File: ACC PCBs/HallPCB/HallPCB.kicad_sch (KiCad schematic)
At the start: 2 parts, among them J1 Conn_01x04_Socket, U1 TLE49643MXTMA1

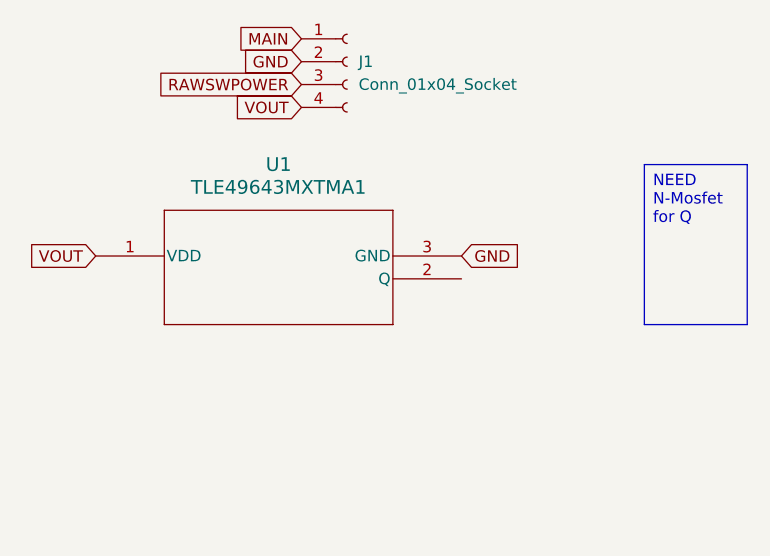
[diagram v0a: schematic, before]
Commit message: All boards should be finished. ACC otw, and an earlier version of the main board otw
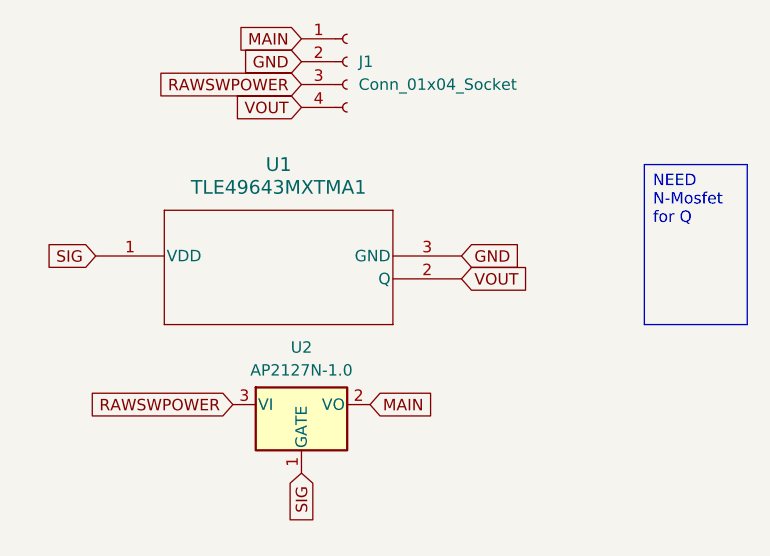
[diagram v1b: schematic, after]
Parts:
- added U2: AP2127N-1.0, Package_TO_SOT_SMD:SOT-23, symbol Regulator_Linear:AP2127N-1.0
- J1: footprint (none) -> Connector_PinHeader_2.54mm:PinHeader_1x04_P2.54mm_Horizontal
- U1: footprint PG-SOT23-3-15_INF -> TLE49643MXTMA1:PG-SOT23-3-15_INF
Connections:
- net MAIN: now also U2.2 (VO)
- net RAWSWPOWER: now also U2.3 (VI)
- net VOUT: now also U1.2 (Q); no longer U1.1 (VDD)
- new net SIG: U1.1 (VDD), U2.1 (GATE)
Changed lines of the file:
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@@
 	(global_label "VOUT"
 		(shape input)
+		(at 160.02 107.95 0)
+		(fields_autoplaced yes)
+		(effects
+			(font
+				(size 1.27 1.27)
+			)
+			(justify left)
+		)
+		(property "Intersheetrefs" "${INTERSHEET_REFS}"
+			(at 167.7224 107.95 0)
+			(effects
+				(font
+					(size 1.27 1.27)
+				)
+				(justify left)
+				(hide yes)
+			)
+		)
+	)
+	(global_label "RAWSWPOWER"
+		(shape input)
+		(at 142.24 86.36 180)
+		(fields_autoplaced yes)
+		(effects
+			(font
+				(size 1.27 1.27)
+			)
+			(justify right)
+		)
+		(property "Intersheetrefs" "${INTERSHEET_REFS}"
+			(at 126.313 86.36 0)
+			(effects
+				(font
+					(size 1.27 1.27)
+				)
+				(justify right)
+				(hide yes)
+			)
+		)
+	)
+	(global_label "MAIN"
+		(shape input)
+		(at 149.86 121.92 0)
+		(fields_autoplaced yes)
+		(effects
+			(font
+				(size 1.27 1.27)
+			)
+			(justify left)
+		)
+		(property "Intersheetrefs" "${INTERSHEET_REFS}"
+			(at 157.3205 121.92 0)
+			(effects
+				(font
+					(size 1.27 1.27)
+				)
+				(justify left)
+				(hide yes)
+			)
+		)
+	)
+	(global_label "RAWSWPOWER"
+		(shape input)
+		(at 134.62 121.92 180)
+		(fields_autoplaced yes)
+		(effects
+			(font
+				(size 1.27 1.27)
+			)
+			(justify right)
+		)
+		(property "Intersheetrefs" "${INTERSHEET_REFS}"
+			(at 118.693 121.92 0)
+			(effects
+				(font
+					(size 1.27 1.27)
+				)
+				(justify right)
+				(hide yes)
+			)
+		)
+	)
+	(global_label "MAIN"
+		(shape input)
+		(at 142.24 81.28 180)
+		(fields_autoplaced yes)
+		(effects
+			(font
+				(size 1.27 1.27)
+			)
+			(justify right)
+		)
+		(property "Intersheetrefs" "${INTERSHEET_REFS}"
+			(at 134.7795 81.28 0)
+			(effects
+				(font
+					(size 1.27 1.27)
+				)
+				(justify right)
+				(hide yes)
+			)
+		)
+	)
+	(global_label "VOUT"
+		(shape input)
+		(at 142.24 88.9 180)
+		(fields_autoplaced yes)
+		(effects
+			(font
+				(size 1.27 1.27)
+			)
+			(justify right)
+		)
+		(property "Intersheetrefs" "${INTERSHEET_REFS}"
+			(at 134.5376 88.9 0)
+			(effects
+				(font
+					(size 1.27 1.27)
+				)
+				(justify right)
+				(hide yes)
+			)
+		)
+	)
+	(global_label "GND"
+		(shape input)
+		(at 142.24 83.82 180)
+		(fields_autoplaced yes)
+		(effects
+			(font
+				(size 1.27 1.27)
+			)
+			(justify right)
+		)
+		(property "Intersheetrefs" "${INTERSHEET_REFS}"
+			(at 135.3843 83.82 0)
+			(effects
+				(font
+					(size 1.27 1.27)
+				)
+				(justify right)
+				(hide yes)
+			)
+		)
+	)
+	(global_label "GND"
+		(shape input)
+		(at 160.02 105.41 0)
+		(fields_autoplaced yes)
+		(effects
+			(font
+				(size 1.27 1.27)
+			)
+			(justify left)
+		)
+		(property "Intersheetrefs" "${INTERSHEET_REFS}"
+			(at 166.8757 105.41 0)
+			(effects
+				(font
+					(size 1.27 1.27)
+				)
+				(justify left)
+				(hide yes)
+			)
+		)
+	)
+	(global_label "SIG"
+		(shape input)
+		(at 142.24 129.54 270)
+		(fields_autoplaced yes)
+		(effects
+			(font
+				(size 1.27 1.27)
+			)
+			(justify right)
+		)
+		(property "Intersheetrefs" "${INTERSHEET_REFS}"
+			(at 142.24 135.6095 90)
+			(effects
+				(font
+					(size 1.27 1.27)
+				)
+				(justify right)
+				(hide yes)
+			)
+		)
+	)
+	(global_label "SIG"
+		(shape input)
 		(at 119.38 105.41 180)
 		(fields_autoplaced yes)
@@
 		)
 		(property "Intersheetrefs" "${INTERSHEET_REFS}"
-			(at 111.6776 105.41 0)
-			(effects
-				(font
-					(size 1.27 1.27)
-				)
-				(justify right)
-				(hide yes)
-			)
-		)
-	)
-	(global_label "RAWSWPOWER"
-		(shape input)
-		(at 142.24 86.36 180)
-		(fields_autoplaced yes)
-		(effects
-			(font
-				(size 1.27 1.27)
-			)
-			(justify right)
-		)
-		(property "Intersheetrefs" "${INTERSHEET_REFS}"
-			(at 126.313 86.36 0)
-			(effects
-				(font
-					(size 1.27 1.27)
-				)
-				(justify right)
-				(hide yes)
-			)
-		)
-	)
-	(global_label "MAIN"
-		(shape input)
-		(at 142.24 81.28 180)
-		(fields_autoplaced yes)
-		(effects
-			(font
-				(size 1.27 1.27)
-			)
-			(justify right)
-		)
-		(property "Intersheetrefs" "${INTERSHEET_REFS}"
-			(at 134.7795 81.28 0)
-			(effects
-				(font
-					(size 1.27 1.27)
-				)
-				(justify right)
-				(hide yes)
-			)
-		)
-	)
-	(global_label "VOUT"
-		(shape input)
-		(at 142.24 88.9 180)
-		(fields_autoplaced yes)
-		(effects
-			(font
-				(size 1.27 1.27)
-			)
-			(justify right)
-		)
-		(property "Intersheetrefs" "${INTERSHEET_REFS}"
-			(at 134.5376 88.9 0)
-			(effects
-				(font
-					(size 1.27 1.27)
-				)
-				(justify right)
-				(hide yes)
-			)
-		)
-	)
-	(global_label "GND"
-		(shape input)
-		(at 142.24 83.82 180)
-		(fields_autoplaced yes)
-		(effects
-			(font
-				(size 1.27 1.27)
-			)
-			(justify right)
-		)
-		(property "Intersheetrefs" "${INTERSHEET_REFS}"
-			(at 135.3843 83.82 0)
-			(effects
-				(font
-					(size 1.27 1.27)
-				)
-				(justify right)
-				(hide yes)
-			)
-		)
-	)
-	(global_label "GND"
-		(shape input)
-		(at 160.02 105.41 0)
-		(fields_autoplaced yes)
-		(effects
-			(font
-				(size 1.27 1.27)
-			)
-			(justify left)
-		)
-		(property "Intersheetrefs" "${INTERSHEET_REFS}"
-			(at 166.8757 105.41 0)
-			(effects
-				(font
-					(size 1.27 1.27)
-				)
-				(justify left)
-				(hide yes)
+			(at 113.3105 105.41 0)
+			(effects
+				(font
+					(size 1.27 1.27)
+				)
+				(justify right)
+				(hide yes)
+			)
+		)
+	)
+	(symbol
+		(lib_id "Regulator_Linear:AP2127N-1.0")
+		(at 142.24 121.92 0)
+		(unit 1)
+		(exclude_from_sim no)
+		(in_bom yes)
+		(on_board yes)
+		(dnp no)
+		(fields_autoplaced yes)
+		(property "Reference" "U2"
+			(at 142.24 115.57 0)
+			(effects
+				(font
+					(size 1.27 1.27)
+				)
+			)
+		)
+		(property "Value" "AP2127N-1.0"
+			(at 142.24 118.11 0)
+			(effects
+				(font
+					(size 1.27 1.27)
+				)
+			)
+		)
+		(property "Footprint" "Package_TO_SOT_SMD:SOT-23"
+			(at 142.24 116.205 0)
+			(effects
+				(font
+					(size 1.27 1.27)
+					(italic yes)
+				)
+				(hide yes)
+			)
+		)
+		(property "Datasheet" "https://www.diodes.com/assets/Datasheets/AP2127.pdf"
+			(at 142.24 121.92 0)
+			(effects
+				(font
+					(size 1.27 1.27)
+				)
+				(hide yes)
+			)
+		)
+		(property "Description" "300mA low dropout linear regulator, shutdown pin, 2.5V-6V input voltage, 1.0V fixed positive output, SOT-23 package"
+			(at 142.24 121.92 0)
+			(effects
+				(font
+					(size 1.27 1.27)
+				)
+				(hide yes)
+			)
+		)
+		(pin "3"
+		)
+		(pin "1"
+		)
+		(pin "2"
+		)
+		(instances
+			(project ""
+				(path "/bca63e1f-d422-43ee-b63a-c2b8269ab195"
+					(reference "U2")
+					(unit 1)
+				)
 			)
 		)
@@
 			)
 		)
-		(property "Footprint" "PG-SOT23-3-15_INF"
+		(property "Footprint" "TLE49643MXTMA1:PG-SOT23-3-15_INF"
 			(at 119.38 105.41 0)
 			(effects
@@
 			)
 		)
-		(property "Footprint" ""
+		(property "Footprint" "Connector_PinHeader_2.54mm:PinHeader_1x04_P2.54mm_Horizontal"
 			(at 147.32 83.82 0)
 			(effects
